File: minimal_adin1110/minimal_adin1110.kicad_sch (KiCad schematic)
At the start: 73 parts, among them J1 CLP-114-02-G-D-BE, J2 CLP-102-02-G-D-BE, J3 CLP-102-02-G-D-BE, J4 CLP-102-02-G-D-BE, J5 CLP-103-02-G-D-BE, U1 ADIN1110CCPZ, Y1 25.0000MHz

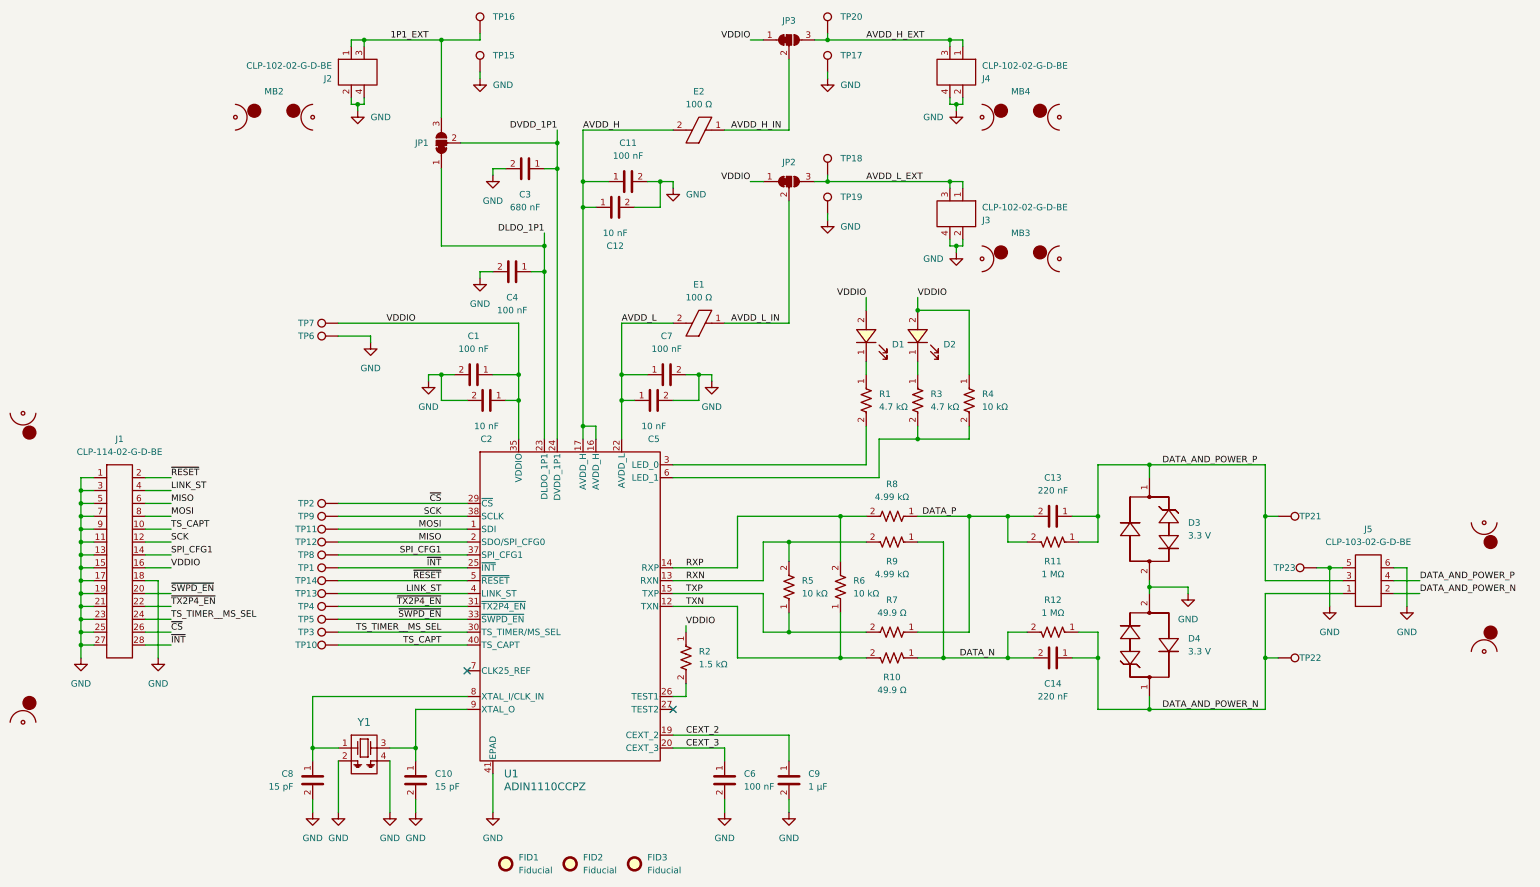
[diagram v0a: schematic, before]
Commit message: development backup
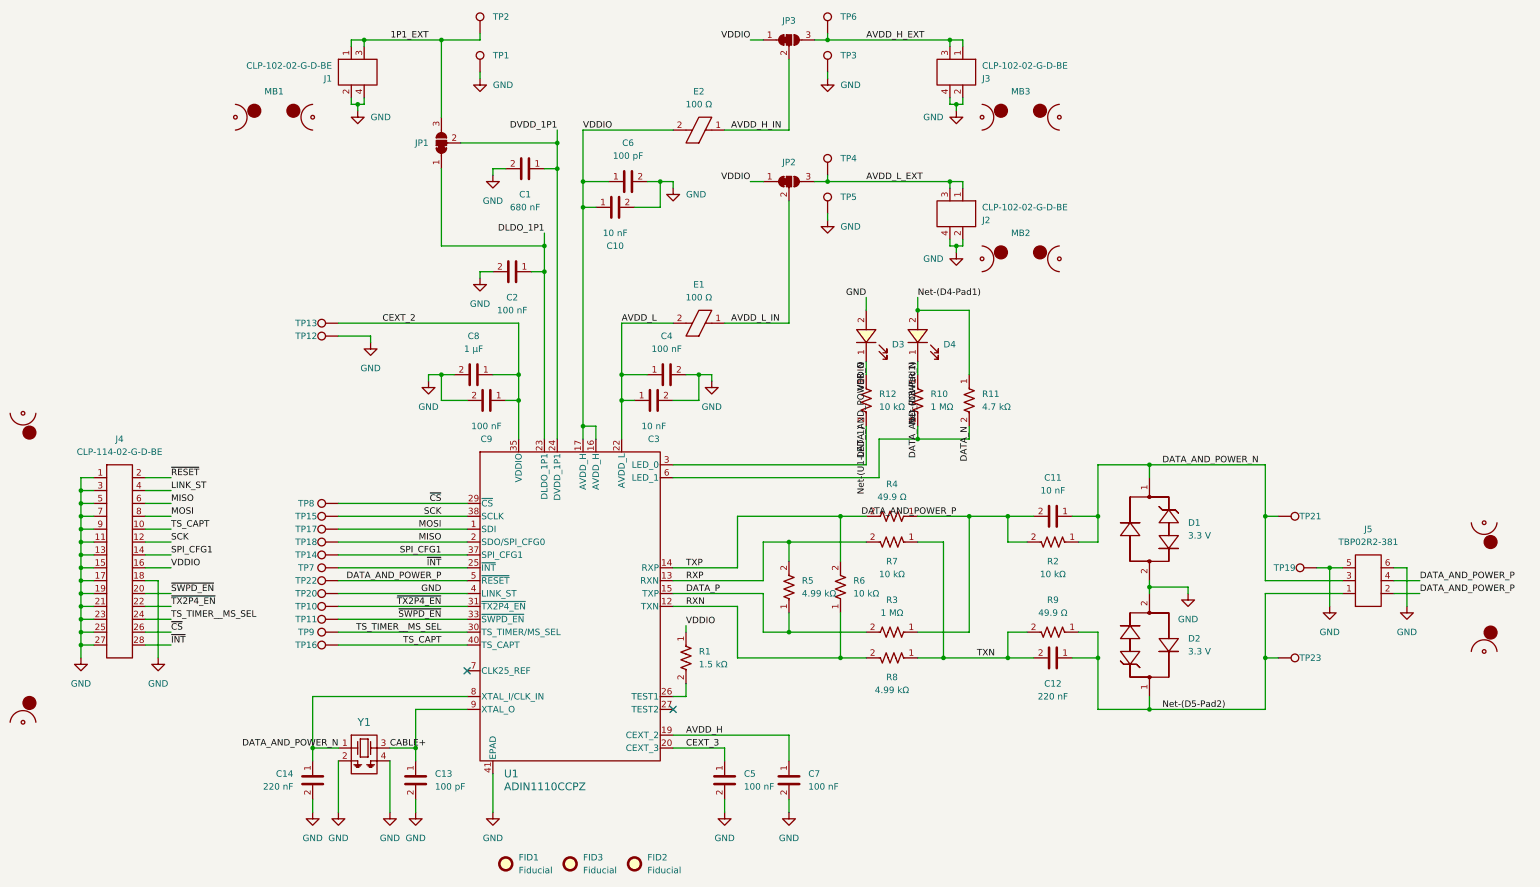
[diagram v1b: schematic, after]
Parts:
- C11: renamed from C13; value 220 nF -> 10 nF; footprint capacitor_footprints:C_0805_2012Metric -> capacitor_footprints:C_0402_1005Metric; 3dviewer Link https://3dviewer.net/index.html#model=https://github.com/ionutms/KiCAD_Symbols_Generator/blob/main/3D_models/C_0805.step -> https://3dviewer.net/index.html#model=https://github.com/ionutms/KiCAD_Symbols_Generator/blob/main/3D_models/C_0402.step; Case Code - in 0805 -> 0402; Case Code - mm 2012 -> 1005; Dielectric X7R -> X7S; MPN C0805C224J1RACTU -> C1005X7S2A103K050BB; Manufacturer Kemet -> TDK; Series C0805C -> C1005X7S2A; Symbol Name C_C0805C224J1RACTU -> C_C1005X7S2A103K050BB; Tolerance 5% -> 10%; Trustedparts Search https://www.trustedparts.com/en/search/C0805C224J1RACTU -> https://www.trustedparts.com/en/search/C1005X7S2A103K050BB; Voltage Rating DC 16 VDC -> 100 VDC
- C13: renamed from C10; value 15 pF -> 100 pF; footprint capacitor_footprints:C_0402_1005Metric -> capacitor_footprints:C_1812_4532Metric; 3dviewer Link https://3dviewer.net/index.html#model=https://github.com/ionutms/KiCAD_Symbols_Generator/blob/main/3D_models/C_0402.step -> https://3dviewer.net/index.html#model=https://github.com/ionutms/KiCAD_Symbols_Generator/blob/main/3D_models/C_1812.step; Case Code - in 0402 -> 1812; Case Code - mm 1005 -> 4532; MPN GCM1555C1H150FA16D -> C1812C101JHGACTU; Manufacturer Murata Electronics -> Kemet; Series GCM1555C1H -> C1812C; Symbol Name C_GCM1555C1H150FA16D -> C_C1812C101JHGACTU; Tolerance 1% -> 5%; Trustedparts Search https://www.trustedparts.com/en/search/GCM1555C1H150FA16D -> https://www.trustedparts.com/en/search/C1812C101JHGACTU; Voltage Rating 50V -> 3kV; Voltage Rating DC 50 VDC -> (none)
- C14: renamed from C8; value 15 pF -> 220 nF; footprint capacitor_footprints:C_0402_1005Metric -> capacitor_footprints:C_0805_2012Metric; 3dviewer Link https://3dviewer.net/index.html#model=https://github.com/ionutms/KiCAD_Symbols_Generator/blob/main/3D_models/C_0402.step -> https://3dviewer.net/index.html#model=https://github.com/ionutms/KiCAD_Symbols_Generator/blob/main/3D_models/C_0805.step; Case Code - in 0402 -> 0805; Case Code - mm 1005 -> 2012; Dielectric C0G (NP0) -> X7R; MPN GCM1555C1H150FA16D -> C0805C224J1RACTU; Manufacturer Murata Electronics -> Kemet; Series GCM1555C1H -> C0805C; Symbol Name C_GCM1555C1H150FA16D -> C_C0805C224J1RACTU; Tolerance 1% -> 5%; Trustedparts Search https://www.trustedparts.com/en/search/GCM1555C1H150FA16D -> https://www.trustedparts.com/en/search/C0805C224J1RACTU; Voltage Rating 50V -> 100V; Voltage Rating DC 50 VDC -> 16 VDC
- C6: renamed from C11; value 100 nF -> 100 pF; footprint capacitor_footprints:C_0402_1005Metric -> capacitor_footprints:C_1812_4532Metric; 3dviewer Link https://3dviewer.net/index.html#model=https://github.com/ionutms/KiCAD_Symbols_Generator/blob/main/3D_models/C_0402.step -> https://3dviewer.net/index.html#model=https://github.com/ionutms/KiCAD_Symbols_Generator/blob/main/3D_models/C_1812.step; Case Code - in 0402 -> 1812; Case Code - mm 1005 -> 4532; Dielectric X7R -> C0G (NP0); MPN GCM155R71H104KE02D -> C1812C101JHGACTU; Manufacturer Murata Electronics -> Kemet; Series GCM155R71H -> C1812C; Symbol Name C_GCM155R71H104KE02D -> C_C1812C101JHGACTU; Tolerance 10% -> 5%; Trustedparts Search https://www.trustedparts.com/en/search/GCM155R71H104KE02D -> https://www.trustedparts.com/en/search/C1812C101JHGACTU; Voltage Rating 50V -> 3kV; Voltage Rating DC 50 VDC -> (none)
- C7: renamed from C9; value 1 µF -> 100 nF; Dielectric X7S -> X7R; MPN C1005X6S1C105K050BC -> GCM155R71H104KE02D; Manufacturer TDK -> Murata Electronics; Series C1005X6S1C -> GCM155R71H; Symbol Name C_C1005X6S1C105K050BC -> C_GCM155R71H104KE02D; Trustedparts Search https://www.trustedparts.com/en/search/C1005X6S1C105K050BC -> https://www.trustedparts.com/en/search/GCM155R71H104KE02D; Voltage Rating 16V -> 50V; Voltage Rating DC 16 VDC -> 50 VDC
- C8: renamed from C1; value 100 nF -> 1 µF; Dielectric X7R -> X7S; MPN GCM155R71H104KE02D -> C1005X6S1C105K050BC; Manufacturer Murata Electronics -> TDK; Series GCM155R71H -> C1005X6S1C; Symbol Name C_GCM155R71H104KE02D -> C_C1005X6S1C105K050BC; Trustedparts Search https://www.trustedparts.com/en/search/GCM155R71H104KE02D -> https://www.trustedparts.com/en/search/C1005X6S1C105K050BC; Voltage Rating 50V -> 16V; Voltage Rating DC 50 VDC -> 16 VDC
- C9: renamed from C2; value 10 nF -> 100 nF; Dielectric X7S -> X7R; MPN C1005X7S2A103K050BB -> GCM155R71H104KE02D; Manufacturer TDK -> Murata Electronics; Series C1005X7S2A -> GCM155R71H; Symbol Name C_C1005X7S2A103K050BB -> C_GCM155R71H104KE02D; Trustedparts Search https://www.trustedparts.com/en/search/C1005X7S2A103K050BB -> https://www.trustedparts.com/en/search/GCM155R71H104KE02D; Voltage Rating 100V -> 50V; Voltage Rating DC 100 VDC -> 50 VDC
- D2: renamed from D4; Diode Type Unidirectional TVS -> Bidirectional TVS; MPN SP4020-01FTG -> SP4020-01FTG-C; Series SP4020-01FTG -> SP4020-01FTG-C; Symbol Name D_SP4020-01FTG -> D_SP4020-01FTG-C; Trustedparts Search https://www.trustedparts.com/en/search/SP4020-01FTG -> https://www.trustedparts.com/en/search/SP4020-01FTG-C
- D3: renamed from D1; value 1.8 V -> 3.3 V; footprint diode_footprints:LED_GREEN_0402_1005Metric -> diode_footprints:SOD323; Diode Type Green LED -> Unidirectional TVS; MPN APHHS1005CGCK -> SP4020-01FTG; Manufacturer Kingbright -> Littelfuse; Maximum DC Current (A) 0.03 -> 0.0; Series APHHS1005CGCK -> SP4020-01FTG; Symbol Name D_APHHS1005CGCK -> D_SP4020-01FTG; Trustedparts Search https://www.trustedparts.com/en/search/APHHS1005CGCK -> https://www.trustedparts.com/en/search/SP4020-01FTG
- J5: value CLP-103-02-G-D-BE -> TBP02R2-381; footprint connector_footprints:CLP-103-02-G-D-BE -> connector_footprints:TBP02R2-381-03BE; Color Black -> Blue; Current Rating (A) 5.2 -> 8.0; MPN CLP-103-02-G-D-BE -> TBP02R2-381-03BE; Manufacturer Samtec -> Same Sky; Mounting Style Surface Mount -> Through Hole; Number of Rows 2 -> 1; Pitch (mm) 1.27 -> 3.81; Series CLP-1xx-02-G-D-BE -> TBP02R2-381; Symbol Name J_CLP-103-02-G-D-BE -> J_TBP02R2-381-03BE; Trustedparts Search https://www.trustedparts.com/en/search/CLP-103-02-G-D-BE -> https://www.trustedparts.com/en/search/TBP02R2-381-03BE
- R10: renamed from R3; value 4.7 kΩ -> 1 MΩ; footprint resistor_footprints:R_0402_1005Metric -> resistor_footprints:R_0603_1608Metric; 3dviewer Link https://3dviewer.net/index.html#model=https://github.com/ionutms/KiCAD_Symbols_Generator/blob/main/3D_models/R_0402.step -> https://3dviewer.net/index.html#model=https://github.com/ionutms/KiCAD_Symbols_Generator/blob/main/3D_models/R_0603.step; Case Code - in 0402 -> 0603; Case Code - mm 1005 -> 1608; MPN ERJ-2GEJ472X -> ERJ-3EKF1004V; Series ERJ-2GEJ -> ERJ-3EKF; Symbol Name R_ERJ-2GEJ472X -> R_ERJ-3EKF1004V; Temperature Coefficient 200 ppm/°C -> 100 ppm/°C; Tolerance 5% -> 1%; Trustedparts Search https://www.trustedparts.com/en/search/ERJ-2GEJ472X -> https://www.trustedparts.com/en/search/ERJ-3EKF1004V; Voltage Rating 50V -> 75V
- R11: renamed from R4; value 10 kΩ -> 4.7 kΩ; MPN ERJ-2RKF1002X -> ERJ-2GEJ472X; Series ERJ-2RKF -> ERJ-2GEJ; Symbol Name R_ERJ-2RKF1002X -> R_ERJ-2GEJ472X; Temperature Coefficient 100 ppm/°C -> 200 ppm/°C; Tolerance 1% -> 5%; Trustedparts Search https://www.trustedparts.com/en/search/ERJ-2RKF1002X -> https://www.trustedparts.com/en/search/ERJ-2GEJ472X
- R12: renamed from R1; value 4.7 kΩ -> 10 kΩ; MPN ERJ-2GEJ472X -> ERJ-2RKF1002X; Series ERJ-2GEJ -> ERJ-2RKF; Symbol Name R_ERJ-2GEJ472X -> R_ERJ-2RKF1002X; Temperature Coefficient 200 ppm/°C -> 100 ppm/°C; Tolerance 5% -> 1%; Trustedparts Search https://www.trustedparts.com/en/search/ERJ-2GEJ472X -> https://www.trustedparts.com/en/search/ERJ-2RKF1002X
- R2: renamed from R11; value 1 MΩ -> 10 kΩ; MPN ERJ-3EKF1004V -> ERJ-3EKF1002V; Symbol Name R_ERJ-3EKF1004V -> R_ERJ-3EKF1002V; Trustedparts Search https://www.trustedparts.com/en/search/ERJ-3EKF1004V -> https://www.trustedparts.com/en/search/ERJ-3EKF1002V
- R3: renamed from R7; value 49.9 Ω -> 1 MΩ; MPN ERJ-3EKF49R9V -> ERJ-3EKF1004V; Symbol Name R_ERJ-3EKF49R9V -> R_ERJ-3EKF1004V; Trustedparts Search https://www.trustedparts.com/en/search/ERJ-3EKF49R9V -> https://www.trustedparts.com/en/search/ERJ-3EKF1004V
- R4: renamed from R8; value 4.99 kΩ -> 49.9 Ω; MPN ERJ-3EKF4991V -> ERJ-3EKF49R9V; Symbol Name R_ERJ-3EKF4991V -> R_ERJ-3EKF49R9V; Trustedparts Search https://www.trustedparts.com/en/search/ERJ-3EKF4991V -> https://www.trustedparts.com/en/search/ERJ-3EKF49R9V
- R5: value 10 kΩ -> 4.99 kΩ; MPN ERJ-3EKF1002V -> ERJ-3EKF4991V; Symbol Name R_ERJ-3EKF1002V -> R_ERJ-3EKF4991V; Trustedparts Search https://www.trustedparts.com/en/search/ERJ-3EKF1002V -> https://www.trustedparts.com/en/search/ERJ-3EKF4991V
- R7: renamed from R9; value 4.99 kΩ -> 10 kΩ; MPN ERJ-3EKF4991V -> ERJ-3EKF1002V; Symbol Name R_ERJ-3EKF4991V -> R_ERJ-3EKF1002V; Trustedparts Search https://www.trustedparts.com/en/search/ERJ-3EKF4991V -> https://www.trustedparts.com/en/search/ERJ-3EKF1002V
- R8: renamed from R10; value 49.9 Ω -> 4.99 kΩ; MPN ERJ-3EKF49R9V -> ERJ-3EKF4991V; Symbol Name R_ERJ-3EKF49R9V -> R_ERJ-3EKF4991V; Trustedparts Search https://www.trustedparts.com/en/search/ERJ-3EKF49R9V -> https://www.trustedparts.com/en/search/ERJ-3EKF4991V
- R9: renamed from R12; value 1 MΩ -> 49.9 Ω; MPN ERJ-3EKF1004V -> ERJ-3EKF49R9V; Symbol Name R_ERJ-3EKF1004V -> R_ERJ-3EKF49R9V; Trustedparts Search https://www.trustedparts.com/en/search/ERJ-3EKF1004V -> https://www.trustedparts.com/en/search/ERJ-3EKF49R9V
- renumbered C3 to C1, C12 to C10, C14 to C12, C4 to C2, C5 to C3, C7 to C4, C6 to C5, D3 to D1, D2 to D4, FID3 to FID2, FID2 to FID3, J2 to J1, J3 to J2, J4 to J3, J1 to J4, MB2 to MB1, MB3 to MB2, MB4 to MB3, MB1 to MB4, R2 to R1, TP15 to TP1, TP4 to TP10, TP5 to TP11, TP6 to TP12, TP7 to TP13, TP8 to TP14, TP9 to TP15, TP10 to TP16, TP11 to TP17, TP12 to TP18, TP23 to TP19, TP16 to TP2, TP13 to TP20, TP14 to TP22, TP22 to TP23, TP17 to TP3, TP18 to TP4, TP19 to TP5, TP20 to TP6, TP1 to TP7, TP2 to TP8, TP3 to TP9
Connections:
- net AVDD_H: now also C7.1, U1.19 (CEXT_2); no longer C10.1, C6.1, E2.2, U1.16 (AVDD_H), U1.17 (AVDD_H)
- net CEXT_2: now also C8.1, C9.1, TP13.1, U1.35 (VDDIO); no longer C7.1, U1.19 (CEXT_2)
- net DATA_AND_POWER_N: now also C10.1, C11.1, C14.1, C6.1, D1.1, D3.1, D4.1, E2.2, J4.16, J5.3, JP2.1 (A), JP3.1 (A), R1.1, R10.1, R12.1, R2.1, TP21.1, U1.16 (AVDD_H), U1.17 (AVDD_H), U1.8 (XTAL_I/CLK_IN), Y1.1; no longer C12.1, D2.1, J5.1, J5.2, R9.1, TP23.1
- net DATA_AND_POWER_P: now also C11.2, J5.2, R2.2, R3.1, R4.1, TP22.1, U1.5 (~{RESET}); no longer C11.1, D1.1, J5.3, R2.1, TP21.1
- net DATA_N: now also R10.2, R11.2, U1.6 (LED_1); no longer C12.2, R7.1, R8.1, R9.2
- net DATA_P: now also R3.2, R5.1, U1.15 (TXP); no longer C11.2, R2.2, R3.1, R4.1
- net GND: now also D3.2, TP20.1, U1.4 (LINK_ST)
- net LINK_ST: no longer TP20.1, U1.4 (LINK_ST)
- net RXN: now also R6.1, R8.2, U1.12 (TXN); no longer R5.2, R7.2, U1.13 (RXN)
- net RXP: now also R5.2, R7.2, U1.13 (RXN); no longer R4.2, R6.2, U1.14 (RXP)
- net TXN: now also C12.2, R7.1, R8.1, R9.2; no longer R6.1, R8.2, U1.12 (TXN)
- net TXP: now also R4.2, R6.2, U1.14 (RXP); no longer R3.2, R5.1, U1.15 (TXP)
- net ~{RESET}: no longer TP22.1, U1.5 (~{RESET})
- net Net-(U1-LED_1): now reaches R12.2, U1.3 (LED_0)
- net CABLE+: now reaches C13.1, U1.9 (XTAL_O), Y1.3
- removed net VDDIO: C8.1, C9.1, D3.2, D4.2, J4.16, JP2.1 (A), JP3.1 (A), R1.1, R11.1, TP13.1, U1.35 (VDDIO)
- new net Net-(D4-Pad1): D4.2, R11.1
- new net Net-(D5-Pad2): C12.1, D2.1, J5.1, R9.1, TP23.1

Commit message: Revert "development backup"
This reverts commit 9283c747e1c3676efe85313f236ce4507e137f4e.
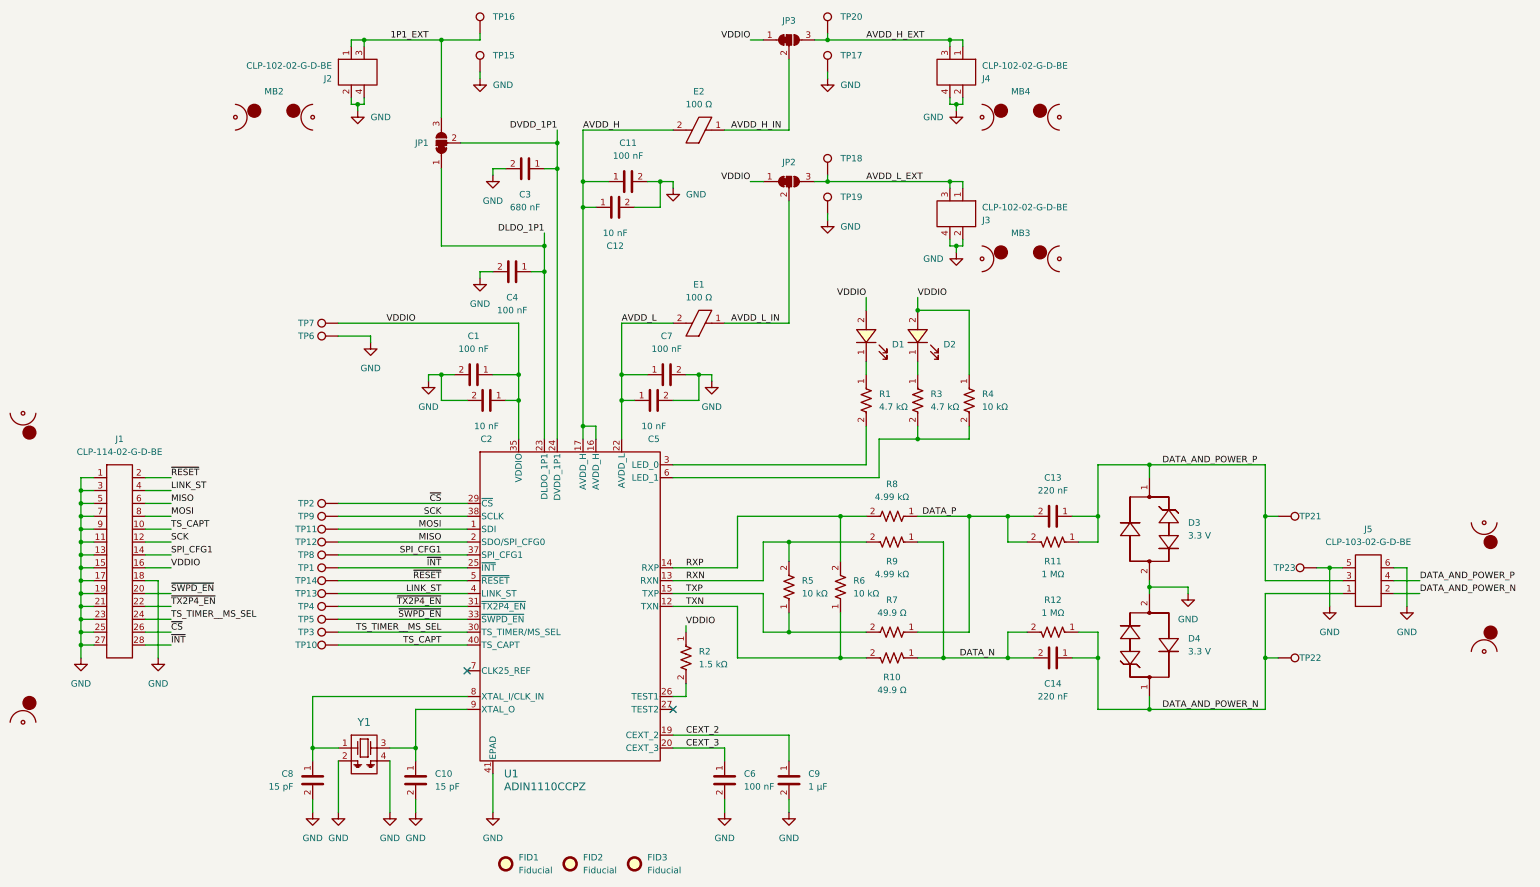
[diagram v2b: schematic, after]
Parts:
- C1: renamed from C8; value 1 µF -> 100 nF; Dielectric X7S -> X7R; MPN C1005X6S1C105K050BC -> GCM155R71H104KE02D; Manufacturer TDK -> Murata Electronics; Series C1005X6S1C -> GCM155R71H; Symbol Name C_C1005X6S1C105K050BC -> C_GCM155R71H104KE02D; Trustedparts Search https://www.trustedparts.com/en/search/C1005X6S1C105K050BC -> https://www.trustedparts.com/en/search/GCM155R71H104KE02D; Voltage Rating 16V -> 50V; Voltage Rating DC 16 VDC -> 50 VDC
- C10: renamed from C13; value 100 pF -> 15 pF; footprint capacitor_footprints:C_1812_4532Metric -> capacitor_footprints:C_0402_1005Metric; 3dviewer Link https://3dviewer.net/index.html#model=https://github.com/ionutms/KiCAD_Symbols_Generator/blob/main/3D_models/C_1812.step -> https://3dviewer.net/index.html#model=https://github.com/ionutms/KiCAD_Symbols_Generator/blob/main/3D_models/C_0402.step; Case Code - in 1812 -> 0402; Case Code - mm 4532 -> 1005; MPN C1812C101JHGACTU -> GCM1555C1H150FA16D; Manufacturer Kemet -> Murata Electronics; Series C1812C -> GCM1555C1H; Symbol Name C_C1812C101JHGACTU -> C_GCM1555C1H150FA16D; Tolerance 5% -> 1%; Trustedparts Search https://www.trustedparts.com/en/search/C1812C101JHGACTU -> https://www.trustedparts.com/en/search/GCM1555C1H150FA16D; Voltage Rating 3kV -> 50V; Voltage Rating DC (none) -> 50 VDC
- C11: renamed from C6; value 100 pF -> 100 nF; footprint capacitor_footprints:C_1812_4532Metric -> capacitor_footprints:C_0402_1005Metric; 3dviewer Link https://3dviewer.net/index.html#model=https://github.com/ionutms/KiCAD_Symbols_Generator/blob/main/3D_models/C_1812.step -> https://3dviewer.net/index.html#model=https://github.com/ionutms/KiCAD_Symbols_Generator/blob/main/3D_models/C_0402.step; Case Code - in 1812 -> 0402; Case Code - mm 4532 -> 1005; Dielectric C0G (NP0) -> X7R; MPN C1812C101JHGACTU -> GCM155R71H104KE02D; Manufacturer Kemet -> Murata Electronics; Series C1812C -> GCM155R71H; Symbol Name C_C1812C101JHGACTU -> C_GCM155R71H104KE02D; Tolerance 5% -> 10%; Trustedparts Search https://www.trustedparts.com/en/search/C1812C101JHGACTU -> https://www.trustedparts.com/en/search/GCM155R71H104KE02D; Voltage Rating 3kV -> 50V; Voltage Rating DC (none) -> 50 VDC
- C13: renamed from C11; value 10 nF -> 220 nF; footprint capacitor_footprints:C_0402_1005Metric -> capacitor_footprints:C_0805_2012Metric; 3dviewer Link https://3dviewer.net/index.html#model=https://github.com/ionutms/KiCAD_Symbols_Generator/blob/main/3D_models/C_0402.step -> https://3dviewer.net/index.html#model=https://github.com/ionutms/KiCAD_Symbols_Generator/blob/main/3D_models/C_0805.step; Case Code - in 0402 -> 0805; Case Code - mm 1005 -> 2012; Dielectric X7S -> X7R; MPN C1005X7S2A103K050BB -> C0805C224J1RACTU; Manufacturer TDK -> Kemet; Series C1005X7S2A -> C0805C; Symbol Name C_C1005X7S2A103K050BB -> C_C0805C224J1RACTU; Tolerance 10% -> 5%; Trustedparts Search https://www.trustedparts.com/en/search/C1005X7S2A103K050BB -> https://www.trustedparts.com/en/search/C0805C224J1RACTU; Voltage Rating DC 100 VDC -> 16 VDC
- C2: renamed from C9; value 100 nF -> 10 nF; Dielectric X7R -> X7S; MPN GCM155R71H104KE02D -> C1005X7S2A103K050BB; Manufacturer Murata Electronics -> TDK; Series GCM155R71H -> C1005X7S2A; Symbol Name C_GCM155R71H104KE02D -> C_C1005X7S2A103K050BB; Trustedparts Search https://www.trustedparts.com/en/search/GCM155R71H104KE02D -> https://www.trustedparts.com/en/search/C1005X7S2A103K050BB; Voltage Rating 50V -> 100V; Voltage Rating DC 50 VDC -> 100 VDC
- C8: renamed from C14; value 220 nF -> 15 pF; footprint capacitor_footprints:C_0805_2012Metric -> capacitor_footprints:C_0402_1005Metric; 3dviewer Link https://3dviewer.net/index.html#model=https://github.com/ionutms/KiCAD_Symbols_Generator/blob/main/3D_models/C_0805.step -> https://3dviewer.net/index.html#model=https://github.com/ionutms/KiCAD_Symbols_Generator/blob/main/3D_models/C_0402.step; Case Code - in 0805 -> 0402; Case Code - mm 2012 -> 1005; Dielectric X7R -> C0G (NP0); MPN C0805C224J1RACTU -> GCM1555C1H150FA16D; Manufacturer Kemet -> Murata Electronics; Series C0805C -> GCM1555C1H; Symbol Name C_C0805C224J1RACTU -> C_GCM1555C1H150FA16D; Tolerance 5% -> 1%; Trustedparts Search https://www.trustedparts.com/en/search/C0805C224J1RACTU -> https://www.trustedparts.com/en/search/GCM1555C1H150FA16D; Voltage Rating 100V -> 50V; Voltage Rating DC 16 VDC -> 50 VDC
- C9: renamed from C7; value 100 nF -> 1 µF; Dielectric X7R -> X7S; MPN GCM155R71H104KE02D -> C1005X6S1C105K050BC; Manufacturer Murata Electronics -> TDK; Series GCM155R71H -> C1005X6S1C; Symbol Name C_GCM155R71H104KE02D -> C_C1005X6S1C105K050BC; Trustedparts Search https://www.trustedparts.com/en/search/GCM155R71H104KE02D -> https://www.trustedparts.com/en/search/C1005X6S1C105K050BC; Voltage Rating 50V -> 16V; Voltage Rating DC 50 VDC -> 16 VDC
- D1: renamed from D3; value 3.3 V -> 1.8 V; footprint diode_footprints:SOD323 -> diode_footprints:LED_GREEN_0402_1005Metric; Diode Type Unidirectional TVS -> Green LED; MPN SP4020-01FTG -> APHHS1005CGCK; Manufacturer Littelfuse -> Kingbright; Maximum DC Current (A) 0.0 -> 0.03; Series SP4020-01FTG -> APHHS1005CGCK; Symbol Name D_SP4020-01FTG -> D_APHHS1005CGCK; Trustedparts Search https://www.trustedparts.com/en/search/SP4020-01FTG -> https://www.trustedparts.com/en/search/APHHS1005CGCK
- D4: renamed from D2; Diode Type Bidirectional TVS -> Unidirectional TVS; MPN SP4020-01FTG-C -> SP4020-01FTG; Series SP4020-01FTG-C -> SP4020-01FTG; Symbol Name D_SP4020-01FTG-C -> D_SP4020-01FTG; Trustedparts Search https://www.trustedparts.com/en/search/SP4020-01FTG-C -> https://www.trustedparts.com/en/search/SP4020-01FTG
- J5: value TBP02R2-381 -> CLP-103-02-G-D-BE; footprint connector_footprints:TBP02R2-381-03BE -> connector_footprints:CLP-103-02-G-D-BE; Color Blue -> Black; Current Rating (A) 8.0 -> 5.2; MPN TBP02R2-381-03BE -> CLP-103-02-G-D-BE; Manufacturer Same Sky -> Samtec; Mounting Style Through Hole -> Surface Mount; Number of Rows 1 -> 2; Pitch (mm) 3.81 -> 1.27; Series TBP02R2-381 -> CLP-1xx-02-G-D-BE; Symbol Name J_TBP02R2-381-03BE -> J_CLP-103-02-G-D-BE; Trustedparts Search https://www.trustedparts.com/en/search/TBP02R2-381-03BE -> https://www.trustedparts.com/en/search/CLP-103-02-G-D-BE
- R1: renamed from R12; value 10 kΩ -> 4.7 kΩ; MPN ERJ-2RKF1002X -> ERJ-2GEJ472X; Series ERJ-2RKF -> ERJ-2GEJ; Symbol Name R_ERJ-2RKF1002X -> R_ERJ-2GEJ472X; Temperature Coefficient 100 ppm/°C -> 200 ppm/°C; Tolerance 1% -> 5%; Trustedparts Search https://www.trustedparts.com/en/search/ERJ-2RKF1002X -> https://www.trustedparts.com/en/search/ERJ-2GEJ472X
- R10: renamed from R8; value 4.99 kΩ -> 49.9 Ω; MPN ERJ-3EKF4991V -> ERJ-3EKF49R9V; Symbol Name R_ERJ-3EKF4991V -> R_ERJ-3EKF49R9V; Trustedparts Search https://www.trustedparts.com/en/search/ERJ-3EKF4991V -> https://www.trustedparts.com/en/search/ERJ-3EKF49R9V
- R11: renamed from R2; value 10 kΩ -> 1 MΩ; MPN ERJ-3EKF1002V -> ERJ-3EKF1004V; Symbol Name R_ERJ-3EKF1002V -> R_ERJ-3EKF1004V; Trustedparts Search https://www.trustedparts.com/en/search/ERJ-3EKF1002V -> https://www.trustedparts.com/en/search/ERJ-3EKF1004V
- R12: renamed from R9; value 49.9 Ω -> 1 MΩ; MPN ERJ-3EKF49R9V -> ERJ-3EKF1004V; Symbol Name R_ERJ-3EKF49R9V -> R_ERJ-3EKF1004V; Trustedparts Search https://www.trustedparts.com/en/search/ERJ-3EKF49R9V -> https://www.trustedparts.com/en/search/ERJ-3EKF1004V
- R3: renamed from R10; value 1 MΩ -> 4.7 kΩ; footprint resistor_footprints:R_0603_1608Metric -> resistor_footprints:R_0402_1005Metric; 3dviewer Link https://3dviewer.net/index.html#model=https://github.com/ionutms/KiCAD_Symbols_Generator/blob/main/3D_models/R_0603.step -> https://3dviewer.net/index.html#model=https://github.com/ionutms/KiCAD_Symbols_Generator/blob/main/3D_models/R_0402.step; Case Code - in 0603 -> 0402; Case Code - mm 1608 -> 1005; MPN ERJ-3EKF1004V -> ERJ-2GEJ472X; Series ERJ-3EKF -> ERJ-2GEJ; Symbol Name R_ERJ-3EKF1004V -> R_ERJ-2GEJ472X; Temperature Coefficient 100 ppm/°C -> 200 ppm/°C; Tolerance 1% -> 5%; Trustedparts Search https://www.trustedparts.com/en/search/ERJ-3EKF1004V -> https://www.trustedparts.com/en/search/ERJ-2GEJ472X; Voltage Rating 75V -> 50V
- R4: renamed from R11; value 4.7 kΩ -> 10 kΩ; MPN ERJ-2GEJ472X -> ERJ-2RKF1002X; Series ERJ-2GEJ -> ERJ-2RKF; Symbol Name R_ERJ-2GEJ472X -> R_ERJ-2RKF1002X; Temperature Coefficient 200 ppm/°C -> 100 ppm/°C; Tolerance 5% -> 1%; Trustedparts Search https://www.trustedparts.com/en/search/ERJ-2GEJ472X -> https://www.trustedparts.com/en/search/ERJ-2RKF1002X
- R5: value 4.99 kΩ -> 10 kΩ; MPN ERJ-3EKF4991V -> ERJ-3EKF1002V; Symbol Name R_ERJ-3EKF4991V -> R_ERJ-3EKF1002V; Trustedparts Search https://www.trustedparts.com/en/search/ERJ-3EKF4991V -> https://www.trustedparts.com/en/search/ERJ-3EKF1002V
- R7: renamed from R3; value 1 MΩ -> 49.9 Ω; MPN ERJ-3EKF1004V -> ERJ-3EKF49R9V; Symbol Name R_ERJ-3EKF1004V -> R_ERJ-3EKF49R9V; Trustedparts Search https://www.trustedparts.com/en/search/ERJ-3EKF1004V -> https://www.trustedparts.com/en/search/ERJ-3EKF49R9V
- R8: renamed from R4; value 49.9 Ω -> 4.99 kΩ; MPN ERJ-3EKF49R9V -> ERJ-3EKF4991V; Symbol Name R_ERJ-3EKF49R9V -> R_ERJ-3EKF4991V; Trustedparts Search https://www.trustedparts.com/en/search/ERJ-3EKF49R9V -> https://www.trustedparts.com/en/search/ERJ-3EKF4991V
- R9: renamed from R7; value 10 kΩ -> 4.99 kΩ; MPN ERJ-3EKF1002V -> ERJ-3EKF4991V; Symbol Name R_ERJ-3EKF1002V -> R_ERJ-3EKF4991V; Trustedparts Search https://www.trustedparts.com/en/search/ERJ-3EKF1002V -> https://www.trustedparts.com/en/search/ERJ-3EKF4991V
- renumbered C10 to C12, C12 to C14, C1 to C3, C2 to C4, C3 to C5, C5 to C6, C4 to C7, D4 to D2, D1 to D3, FID3 to FID2, FID2 to FID3, J4 to J1, J1 to J2, J2 to J3, J3 to J4, MB4 to MB1, MB1 to MB2, MB2 to MB3, MB3 to MB4, R1 to R2, TP7 to TP1, TP16 to TP10, TP17 to TP11, TP18 to TP12, TP20 to TP13, TP22 to TP14, TP1 to TP15, TP2 to TP16, TP3 to TP17, TP4 to TP18, TP5 to TP19, TP8 to TP2, TP6 to TP20, TP23 to TP22, TP19 to TP23, TP9 to TP3, TP10 to TP4, TP11 to TP5, TP12 to TP6, TP13 to TP7, TP14 to TP8, TP15 to TP9
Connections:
- net Net-(D5-Pad2) is gone; now on net DATA_AND_POWER_N: C14.1, D4.1, J5.1, R12.1, TP22.1
- net AVDD_H: now also C11.1, C12.1, E2.2, U1.16 (AVDD_H), U1.17 (AVDD_H); no longer C9.1, U1.19 (CEXT_2)
- net CEXT_2: now also C9.1, U1.19 (CEXT_2); no longer C1.1, C2.1, TP7.1, U1.35 (VDDIO)
- net DATA_AND_POWER_N: now also J5.2; no longer C11.1, C12.1, C13.1, C8.1, D1.1, D2.1, D3.1, E2.2, J1.16, J5.3, JP2.1 (A), JP3.1 (A), R1.1, R11.1, R2.1, R3.1, TP21.1, U1.16 (AVDD_H), U1.17 (AVDD_H), U1.8 (XTAL_I/CLK_IN), Y1.1
- net DATA_AND_POWER_P: now also C13.1, D3.1, J5.3, R11.1, TP21.1; no longer C13.2, J5.2, R11.2, R7.1, R8.1, TP14.1, U1.5 (~{RESET})
- net DATA_N: now also C14.2, R10.1, R12.2, R9.1; no longer R3.2, R4.2, U1.6 (LED_1)
- net DATA_P: now also C13.2, R11.2, R7.1, R8.1; no longer R5.1, R7.2, U1.15 (TXP)
- net GND: no longer D1.2, TP13.1, U1.4 (LINK_ST)
- net LINK_ST: now also TP13.1, U1.4 (LINK_ST)
- net RXN: now also R5.2, R9.2, U1.13 (RXN); no longer R10.2, R6.1, U1.12 (TXN)
- net RXP: now also R6.2, R8.2, U1.14 (RXP); no longer R5.2, R9.2, U1.13 (RXN)
- net TXN: now also R10.2, R6.1, U1.12 (TXN); no longer C14.2, R10.1, R12.2, R9.1
- net TXP: now also R5.1, R7.2, U1.15 (TXP); no longer R6.2, R8.2, U1.14 (RXP)
- net ~{RESET}: now also TP14.1, U1.5 (~{RESET})
- net CABLE+: no longer names the net of C10.1, U1.9 (XTAL_O), Y1.3
- net Net-(D4-Pad1) renamed VDDIO
- net VDDIO: now also C1.1, C2.1, D1.2, J1.16, JP2.1 (A), JP3.1 (A), R2.1, TP7.1, U1.35 (VDDIO)
- net Net-(U1-LED_1): no longer names the net of R1.2, U1.3 (LED_0)
- new net: R3.2, R4.2, U1.6 (LED_1)
- new net: C8.1, U1.8 (XTAL_I/CLK_IN), Y1.1
- new net: D1.1, R1.1
- new net: D2.1, R3.1
